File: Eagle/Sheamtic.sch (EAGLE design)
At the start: 19 parts, among them IC1 PIC16F874P

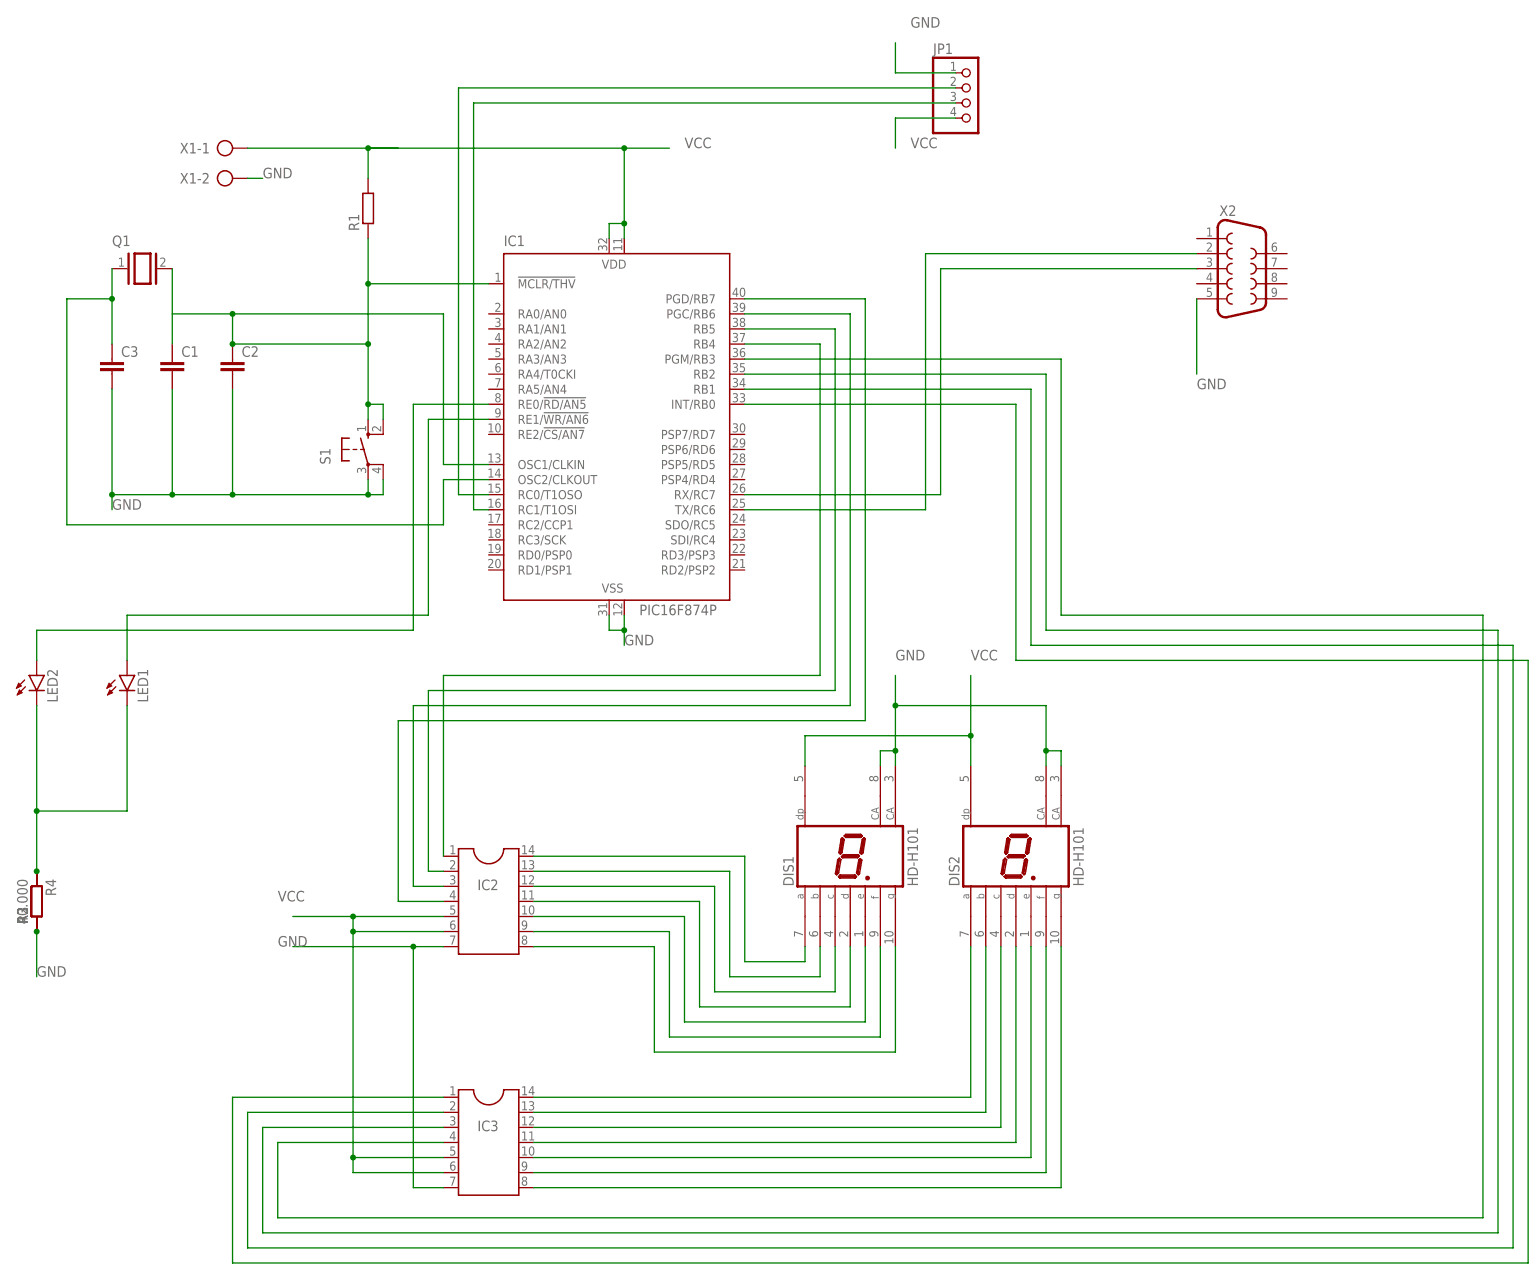
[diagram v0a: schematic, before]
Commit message: eagle update
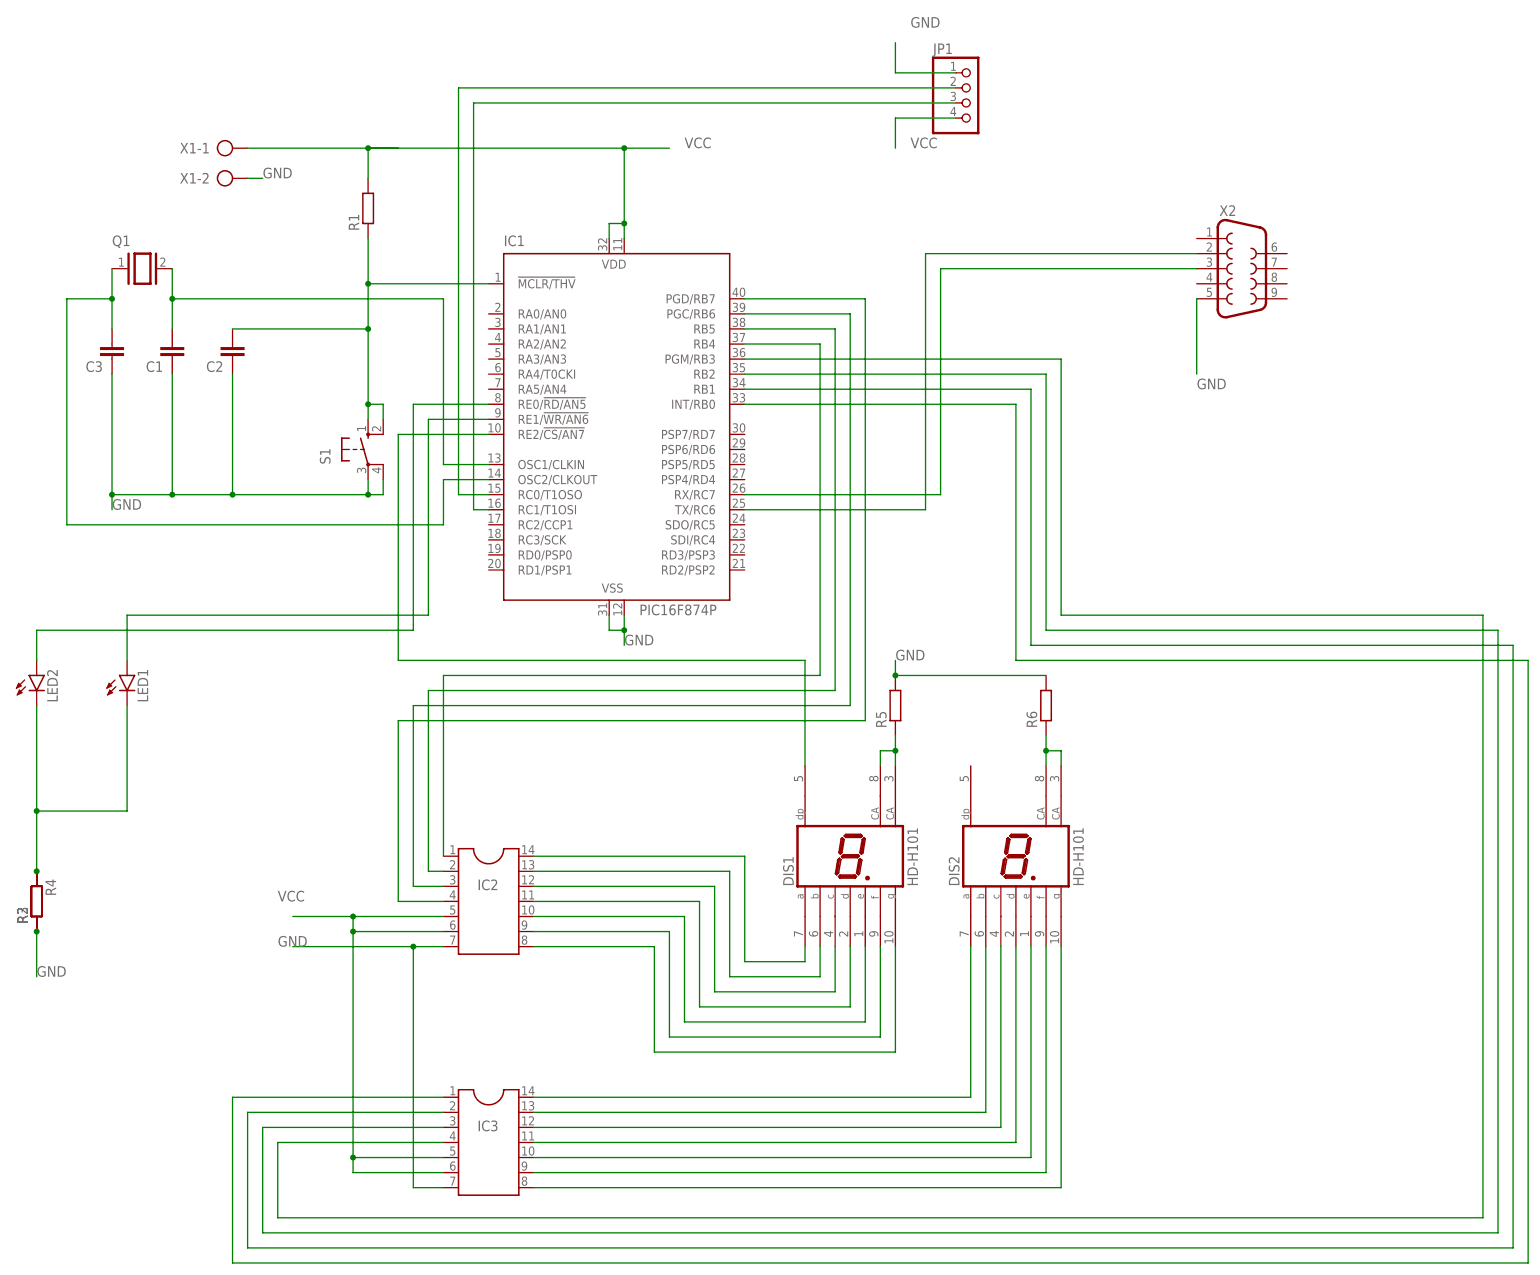
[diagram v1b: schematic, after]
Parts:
- added R5, R6: (no value), rcl:R-EU_0204/7
- R4: value 40.000 -> (none)
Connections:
- new net N$34: DIS1.DP, IC1.RE2/!CS/AN7
- new net N$35: DIS2.CA, DIS2.CA@1, R6.1
- net GND: now also C1.1, C2.1, C3.1, R5.1, R5.2, R6.2; no longer C1.2, C2.2, C3.2, DIS2.CA, DIS2.CA@1
- net N$2: now also C2.2; no longer C2.1, IC1.OSC1/CLKIN
- net N$5: now also C3.2; no longer C3.1
- net N$9: now also C1.2, IC1.OSC1/CLKIN; no longer C1.1
- net VCC: no longer DIS1.DP, DIS2.DP
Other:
- moved on the sheet: C1, C2, C3
